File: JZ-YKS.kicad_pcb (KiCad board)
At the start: 2 copper layers, 50 x 50 mm, 58 parts, among them U3 VREG-DUAL

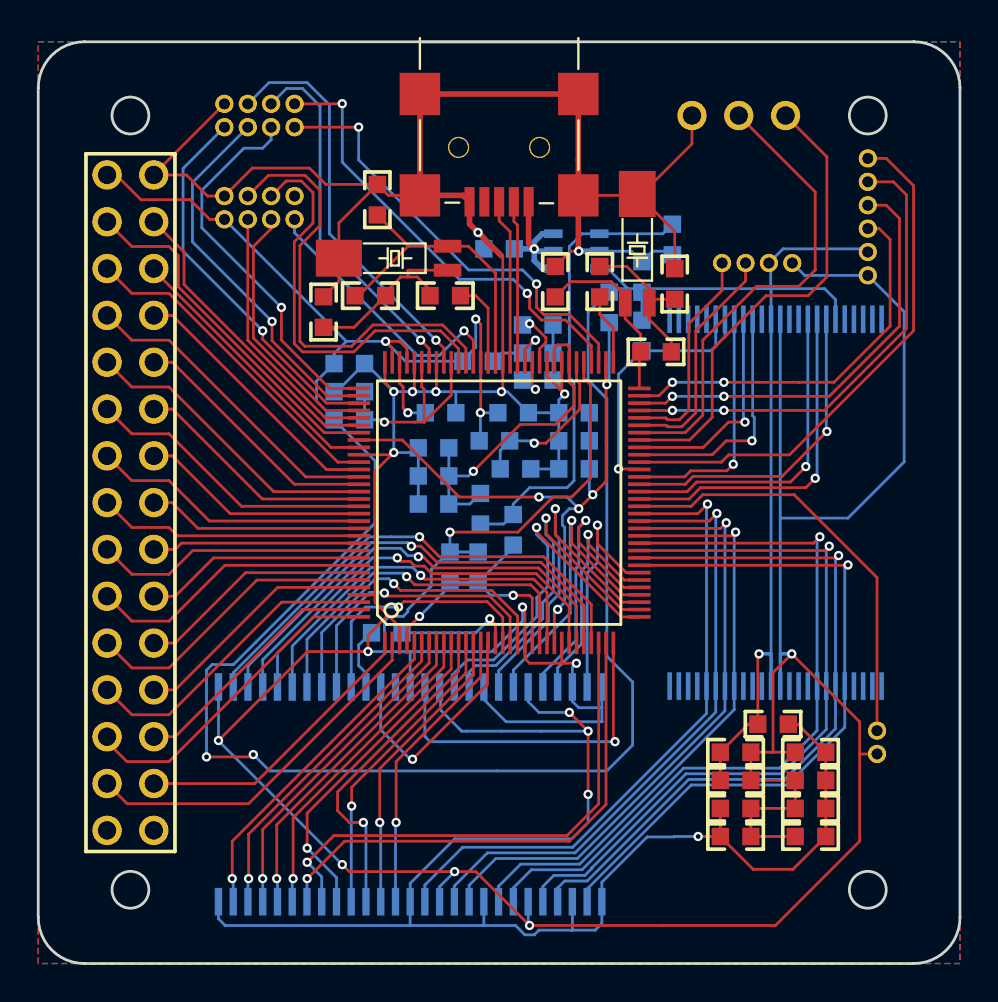
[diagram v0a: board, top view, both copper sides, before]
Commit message: rev.A that was actualy manufactured
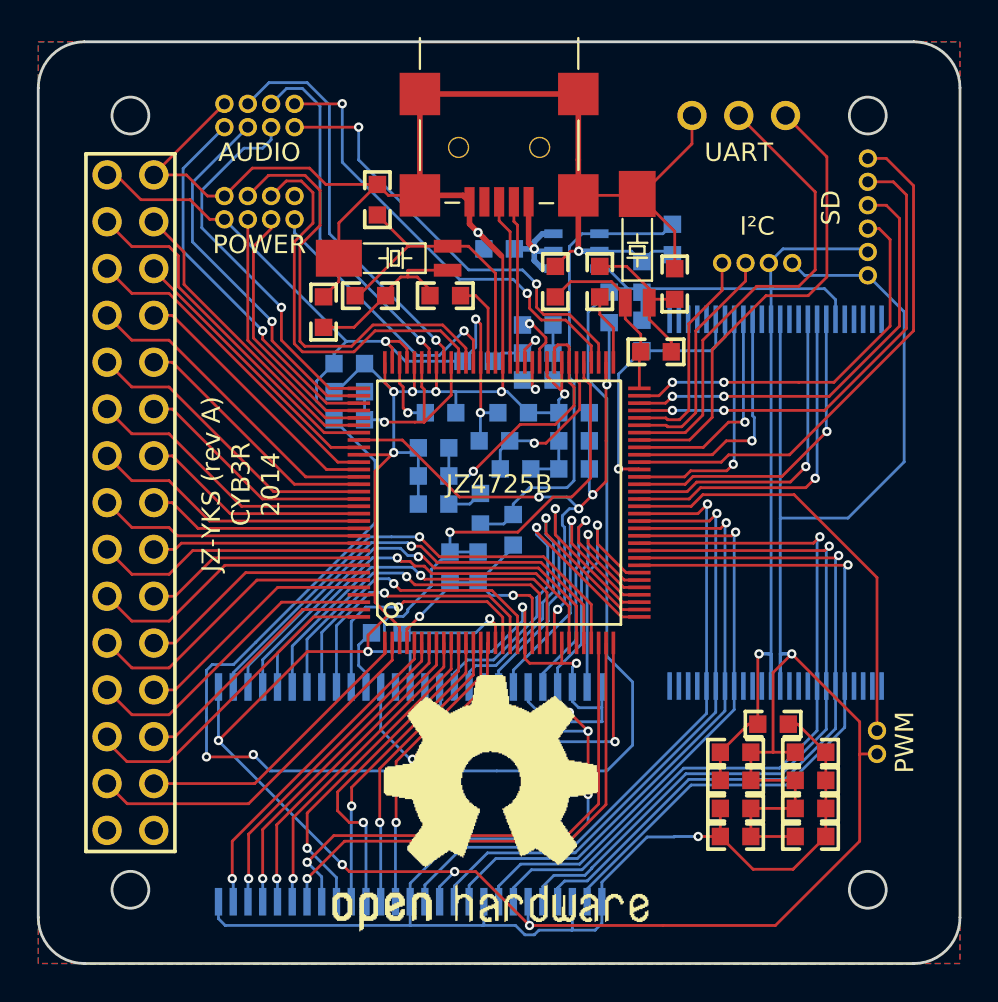
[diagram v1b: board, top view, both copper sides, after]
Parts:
- added G***: LOGO, OSHWLOGO0.75IN, F.Cu at (125.0, 107.0)
- C18: renamed from ?; value (none) -> 22pF
- IC1: renamed from ?; value (none) -> JZ4725
- U1: renamed from ?; value (none) -> PINHEAD30
- U10: renamed from ?; value (none) -> PINHEAD2
- U2, U9: renamed from ?; value (none) -> PINHEAD8
- U4: renamed from ?; value (none) -> HY27UG088G5M
- U5: renamed from ?; value (none) -> P3V56S40ETP-G6
- U6: renamed from ?; value (none) -> PINHEAD6
- U7: renamed from ?; value (none) -> PINHEAD4
- U8: renamed from ?; value (none) -> PINHEAD3
- gave numbers to parts that had none: 2
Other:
- board text added: "AUDIO"
- board text added: "I²C"
- board text added: "JZ-YKS (rev A) CYB3R 2014"
- board text added: "JZ4725B"
- board text added: "NAND FLASH"
- board text added: "POWER"
- board text added: "PWM"
- board text added: "RAM"
- board text added: "SD"
- board text added: "UART"

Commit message: final fixes for rev.A
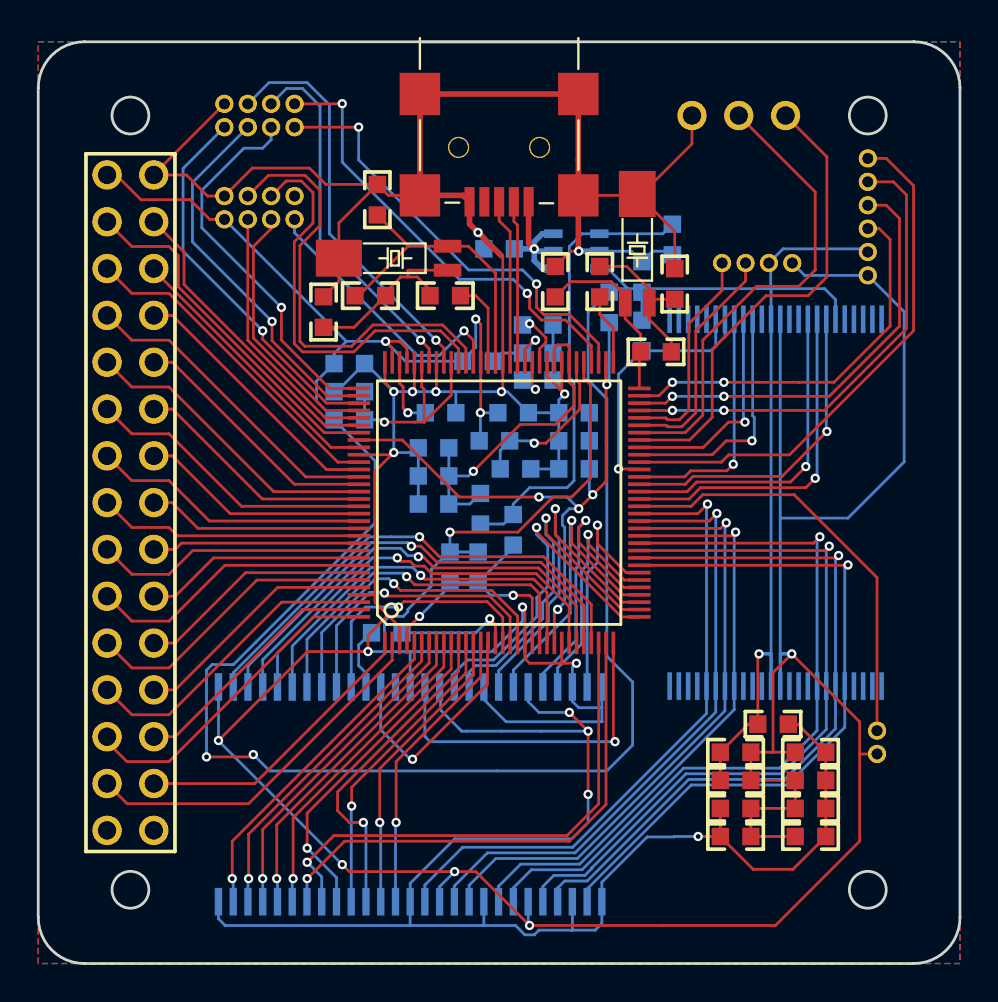
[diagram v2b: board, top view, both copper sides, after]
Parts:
- removed G***: LOGO, OSHWLOGO0.75IN
- ?: renamed from U9; value PINHEAD8 -> (none)
- ?: renamed from U4; value HY27UG088G5M -> (none)
- ?: renamed from U5; value P3V56S40ETP-G6 -> (none)
- ?: renamed from U1; value PINHEAD30 -> (none)
- ?: renamed from U2; value PINHEAD8 -> (none)
- ?: renamed from U10; value PINHEAD2 -> (none)
- ?: renamed from U6; value PINHEAD6 -> (none)
- ?: renamed from U7; value PINHEAD4 -> (none)
- ?: renamed from U8; value PINHEAD3 -> (none)
- ?: renamed from IC1; value JZ4725 -> (none)
- ?: renamed from C18; value 22pF -> (none)
- renumbered X1 to ?, J1 to ?
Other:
- board text removed: "AUDIO"
- board text removed: "I²C"
- board text removed: "JZ-YKS (rev A) CYB3R 2014"
- board text removed: "JZ4725B"
- board text removed: "NAND FLASH"
- board text removed: "POWER"
- board text removed: "PWM"
- board text removed: "RAM"
- board text removed: "SD"
- board text removed: "UART"
